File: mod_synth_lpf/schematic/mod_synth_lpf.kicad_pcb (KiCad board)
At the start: 2 copper layers, 41.3 x 109.2 mm, 42 parts, among them J1 AudioJack2, J2 AudioJack2, J3 AudioJack2, J4 Conn_02x08_Odd_Even, J5 Conn_01x07_Female, J6 Conn_01x07_Male, J7 Conn_01x07_Female, J8 Conn_01x07_Male, Q1 BC558, Q2 BC558, SW1 SW_DPDT_x2, U1 TL074, U2 LM13700

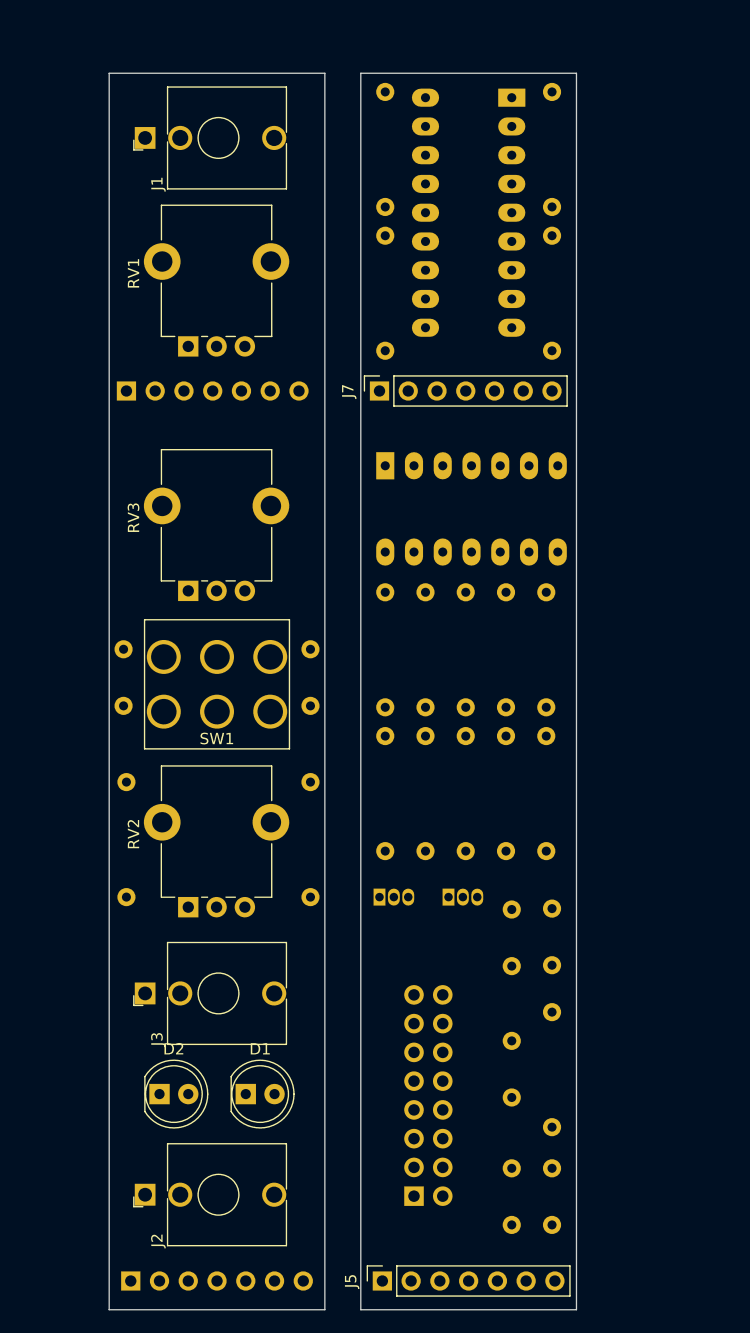
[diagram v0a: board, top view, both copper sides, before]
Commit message: Try to clean up layout
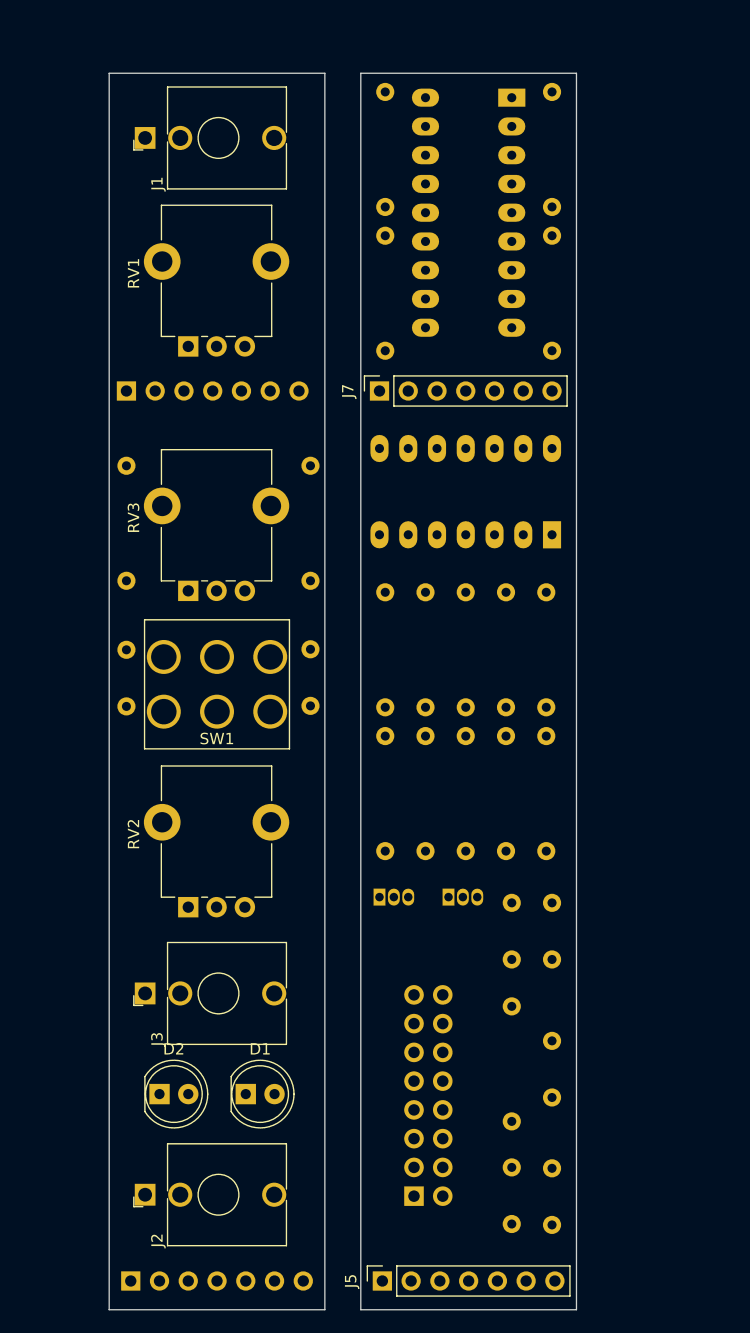
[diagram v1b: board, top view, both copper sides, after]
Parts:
- moved R8 55.4 mm to (106.2, 98.6), turned to 90 degrees
- moved R5 38.1 mm to (72.6, 64.5), turned to 270 degrees
- moved R9 34.8 mm to (110.2, 44.2)
- moved R2 27.9 mm to (88.9, 74.7)
- moved R1 23.9 mm to (109.7, 75.7), turned to 270 degrees
- moved U1 15.9 mm to (110.2, 70.6), turned to 90 degrees
- moved R11 14.7 mm to (95.5, 44.2)
- moved R3 14.6 mm to (99.1, 85.9)
- moved R17 12.7 mm to (102.6, 98.6)
- moved R6 12.4 mm to (102.6, 75.7), turned to 270 degrees
- moved R10 10.2 mm to (99.1, 88.4), turned to 270 degrees
- moved R13 10.2 mm to (109.7, 88.4), turned to 270 degrees
- moved C6 6.20 mm to (106.7, 126.5), turned to 270 degrees
- moved C2 5.59 mm to (106.7, 103.1), turned to 270 degrees
- moved C4 4.96 mm to (72.6, 80.8), turned to 270 degrees
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
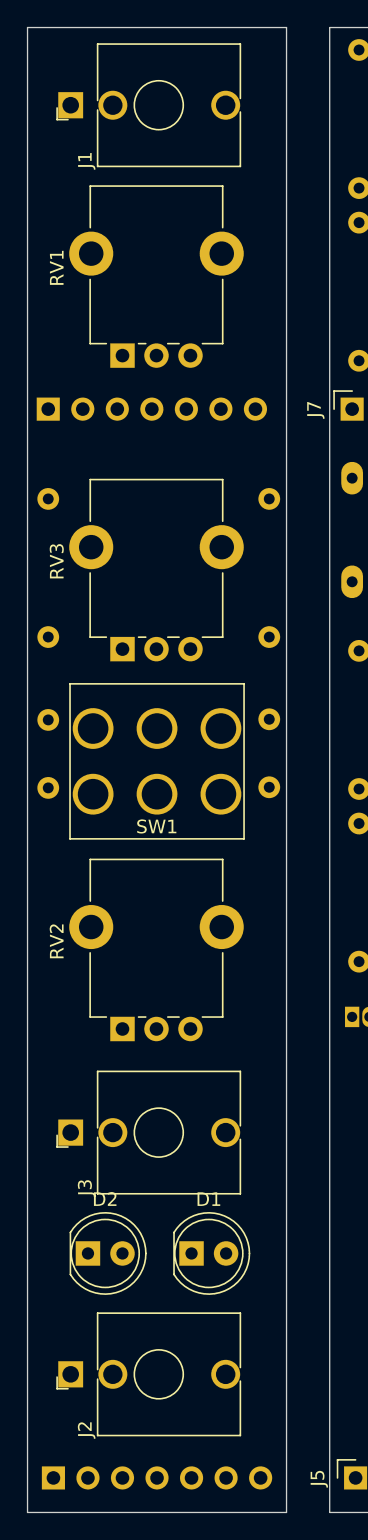
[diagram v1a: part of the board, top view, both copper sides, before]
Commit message: Layout first PCB
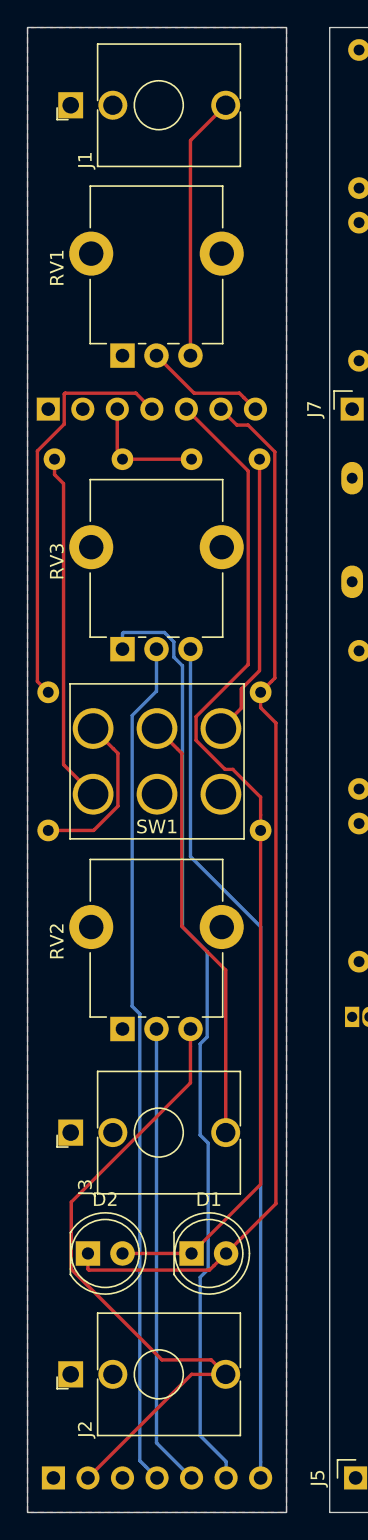
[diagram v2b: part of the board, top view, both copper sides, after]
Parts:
- moved C7 24.8 mm to (83.2, 61.6), turned to 0 degrees
- moved C4 19.9 mm to (78.1, 61.6), turned to 180 degrees
- moved R11 14.7 mm to (110.2, 44.2)
- moved R9 14.7 mm to (95.5, 44.2)
- moved R2 14.2 mm to (88.3, 88.9)
- moved R5 14.2 mm to (72.6, 78.7)
- moved R16 10.2 mm to (95.5, 31.5), turned to 270 degrees
- moved R3 7.11 mm to (106.2, 85.9)
- moved R6 3.56 mm to (99.1, 75.7)
- moved R7 3.56 mm to (102.6, 85.9)
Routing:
- net /INDICATOR_1_PCB_B: track 0.00 -> 78.5 mm
- net /INDICATOR_2_PCB_B: track 0.00 -> 75.1 mm
- net /-12_PCB_B: track 0.00 -> 69.2 mm
- net /+12_PCB_B: track 0.00 -> 63.1 mm
- net /CUT_OFF_PCB_B: track 0.00 -> 62.5 mm
- net /AUDIO_OUT_PCB_B: track 0.00 -> 49.1 mm
- net /RESONANCE_PCB_B: track 0.00 -> 34.1 mm
- net Net-(J3-PadT): track 0.00 -> 31.8 mm
- net /SWB_PCB_B: track 0.00 -> 30.0 mm
- net Net-(C4-Pad2): track 0.00 -> 25.8 mm
- net Net-(C7-Pad2): track 0.00 -> 21.0 mm
- net Net-(J1-PadT): track 0.00 -> 19.5 mm
- net Net-(R5-Pad2): track 0.00 -> 12.3 mm
- net /SWA_PCB_B: track 0.00 -> 8.92 mm
- net /CV_PCB_B: track 0.00 -> 8.91 mm
- added copper zone on B.Cu, net /GND_PCB_B
- added copper zone on F.Cu, net /GND_PCB_B

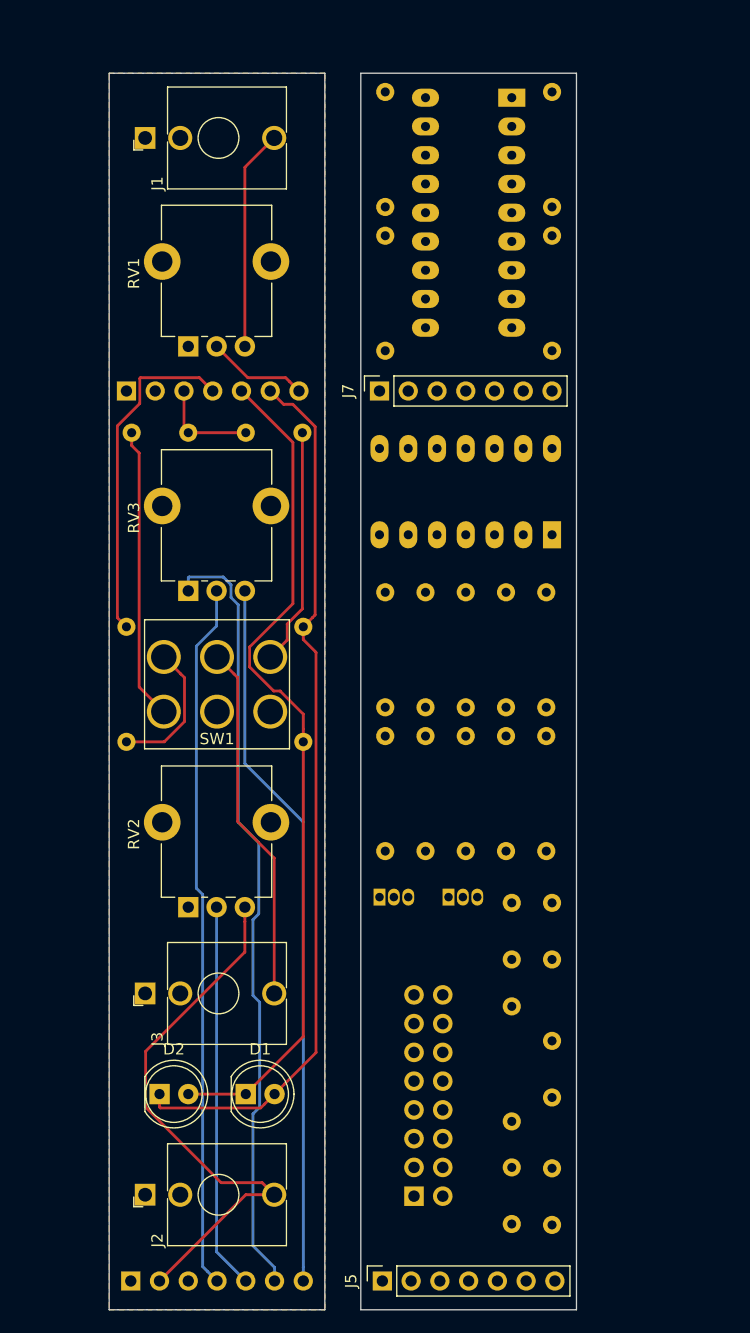
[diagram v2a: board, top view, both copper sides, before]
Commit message: Layout 6hp board
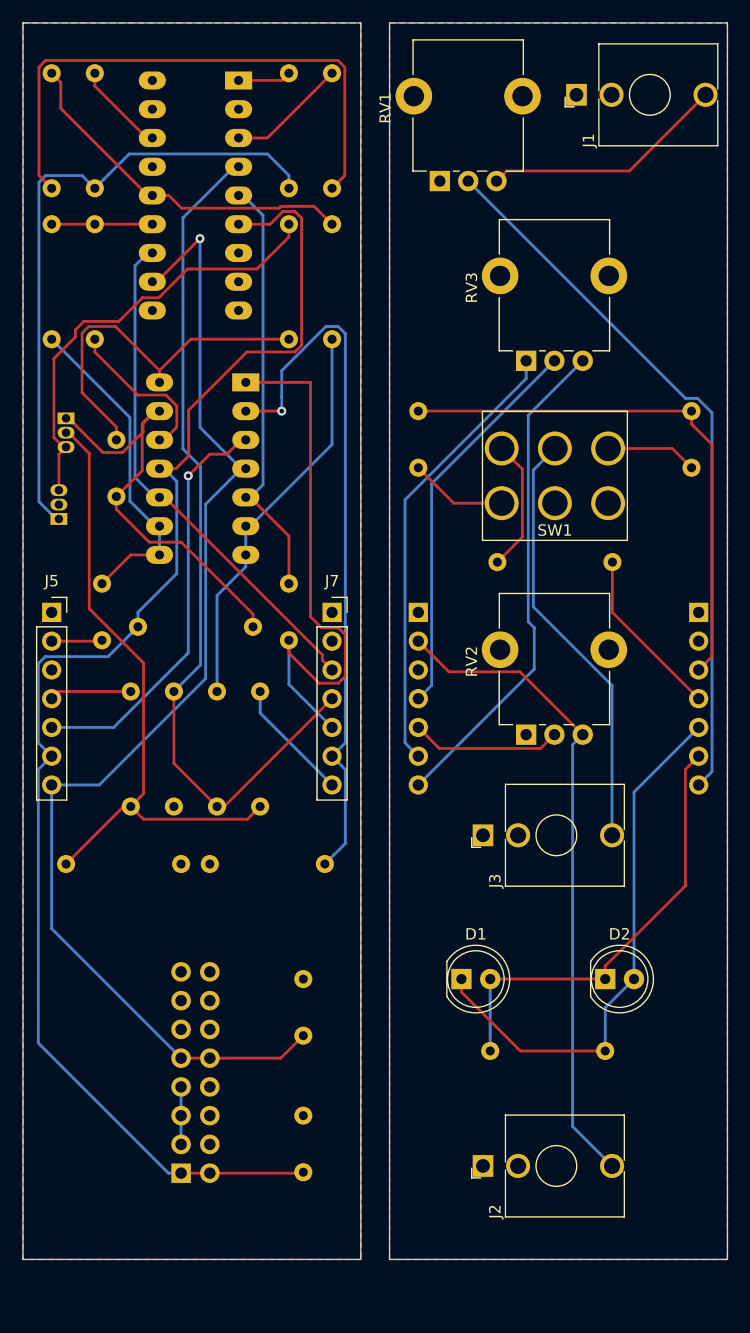
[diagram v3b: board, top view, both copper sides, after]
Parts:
- moved J5 65.9 mm to (66.0, 77.5), turned to 0 degrees
- moved J6 64.3 mm to (98.4, 77.5), turned to 180 degrees
- moved R3 60.9 mm to (66.0, 40.0)
- moved R17 57.5 mm to (87.0, 43.2), turned to 270 degrees
- moved J8 54.2 mm to (123.2, 77.5), turned to 180 degrees
- moved C2 53.8 mm to (71.8, 62.2)
- moved Q2 50.5 mm to (67.3, 60.3), turned to 270 degrees
- moved C3 48.7 mm to (70.5, 74.9)
- moved Q1 48.0 mm to (66.7, 69.2), turned to 90 degrees
- moved C1 46.6 mm to (87.0, 74.9)
- moved R5 43.3 mm to (115.6, 73.0), turned to 180 degrees
- moved R4 41.4 mm to (69.8, 53.3)
- moved R12 41.3 mm to (67.3, 99.7), turned to 0 degrees
- moved D2 40.7 mm to (114.9, 109.9)
- moved C7 39.4 mm to (122.6, 59.7), turned to 270 degrees
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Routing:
- net -12V: track 0.00 -> 127.2 mm
- net +12V: track 0.00 -> 105.8 mm, vias 0 -> 1
- net /SWB_PCB_A: track 0.00 -> 76.1 mm
- net GND: track 0.00 -> 64.0 mm
- net /INDICATOR_1_PCB_A: track 0.00 -> 62.8 mm, vias 0 -> 1
- net Net-(Q2-Pad2): track 0.00 -> 56.6 mm
- net Net-(Q1-Pad1): track 0.00 -> 56.6 mm
- net /CV_PCB_B: track 8.91 -> 63.4 mm
- net /INDICATOR_2_PCB_A: track 0.00 -> 50.6 mm
- net /SWA_PCB_A: track 0.00 -> 45.4 mm
- net /SWA_PCB_B: track 8.92 -> 48.2 mm
- net Net-(Q1-Pad3): track 0.00 -> 39.2 mm
- net /INDICATOR_1_PCB_B: track 78.5 -> 39.6 mm
- net Net-(C2-Pad2): track 0.00 -> 38.6 mm
- net Net-(C1-Pad1): track 0.00 -> 38.1 mm
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- added copper zone on B.Cu, net GND
- added copper zone on F.Cu, net GND
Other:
- board size 41.3 x 109.2 mm -> 62.2 x 109.2 mm
